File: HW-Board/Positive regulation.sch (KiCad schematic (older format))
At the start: 17 parts, among them Q2 Si4435, U2 MCP4725, U3 AD5245, U4 OP07, U5 INA219POS

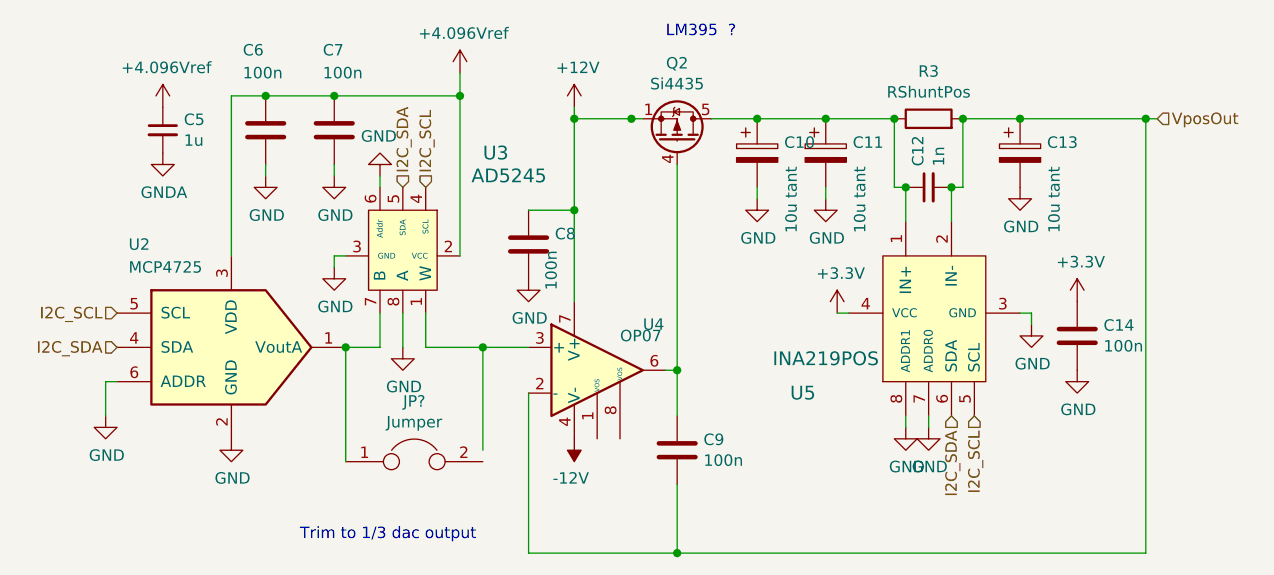
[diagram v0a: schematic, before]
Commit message: sync
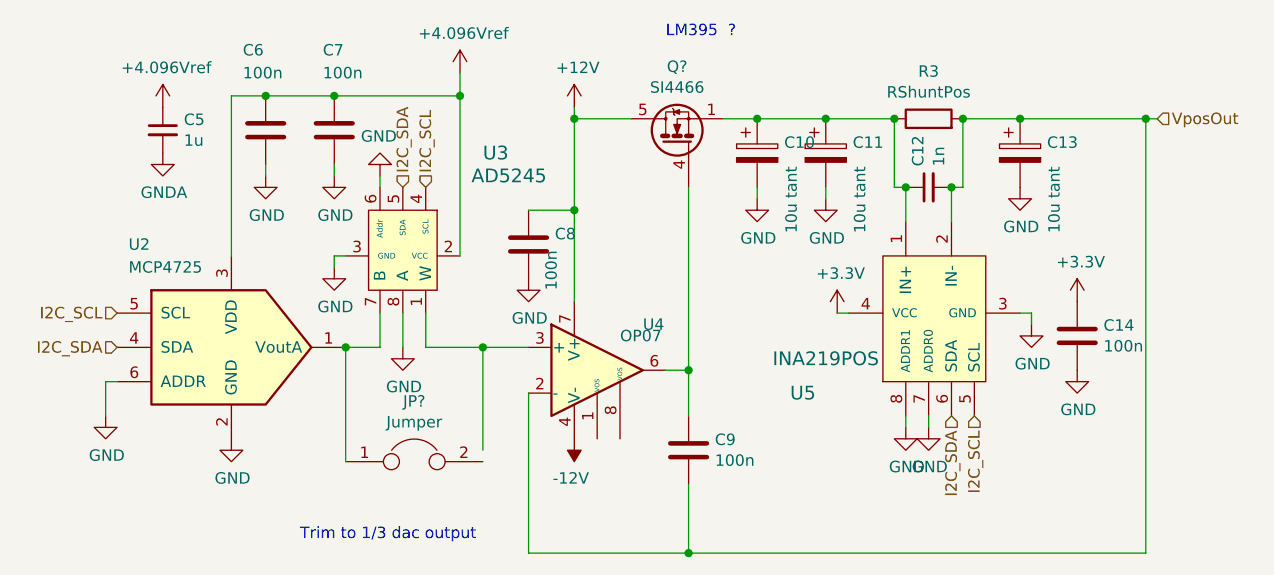
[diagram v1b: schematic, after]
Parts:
- removed Q2: Si4435, Package_SO:SOIC-8_3.9x4.9mm_P1.27mm, symbol BreadbaordPSU-rescue:Si4435-Peters
- added Q?: SI4466, Package_SO:SOIC-8_3.9x4.9mm_P1.27mm, symbol Peters:SI4466
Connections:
- net +12V: now also Q?.5 (D), Q?.6 (D), Q?.7 (D), Q?.8 (D)
- net at C10.1, C11.1, C12.1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: now also Q?.1 (S), Q?.2 (S), Q?.3 (S)
- net at C9.1, U4.6: now also Q?.4 (G)
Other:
- moved on the sheet: C9
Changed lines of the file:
@@
 	5950 2550 5950 2500
 Wire Wire Line
-	6400 3650 6350 3650
+	6450 3650 6350 3650
 Wire Wire Line
 	5750 3750 5750 4450
 Wire Wire Line
-	5750 4450 6400 4450
+	5750 4450 6450 4450
 Wire Wire Line
 	8450 4450 8450 2550
@@
 L Device:C C?
 U 1 1 5CFA023C
-P 6400 4000
+P 6450 4000
 AR Path="/5CFAD453/5CFA023C" Ref="C?"  Part="1"
 AR Path="/5CF8F081/5CFA023C" Ref="C9"  Part="1"
-F 0 "C9" H 6515 4046 50  0000 L CNN
-F 1 "100n" H 6515 3955 50  0000 L CNN
-F 2 "" H 6438 3850 50  0001 C CNN
-F 3 "~" H 6400 4000 50  0001 C CNN
-	1    6400 4000
-	1    0    0    -1
-$EndComp
-Wire Wire Line
-	6400 3850 6400 3650
-Connection ~ 6400 3650
-Wire Wire Line
-	6400 4150 6400 4450
+F 0 "C9" H 6565 4046 50  0000 L CNN
+F 1 "100n" H 6565 3955 50  0000 L CNN
+F 2 "" H 6488 3850 50  0001 C CNN
+F 3 "~" H 6450 4000 50  0001 C CNN
+	1    6450 4000
+	1    0    0    -1
+$EndComp
+Wire Wire Line
+	6450 3850 6450 3650
+Connection ~ 6450 3650
+Wire Wire Line
+	6450 4150 6450 4450
 Wire Wire Line
 	5950 2550 5950 2950
@@
 	3900 3700 3900 3850
 Wire Wire Line
-	6400 4450 8450 4450
-Connection ~ 6400 4450
+	6450 4450 8450 4450
+Connection ~ 6450 4450
 Wire Wire Line
 	7350 2550 7050 2550
@@
 LM395  ?
 Wire Wire Line
-	6400 2750 6400 3650
-Wire Wire Line
-	6550 2550 6750 2550
-Wire Wire Line
-	6200 2550 5950 2550
-Wire Wire Line
-	6250 2550 6200 2550
-Connection ~ 6200 2550
-$Comp
-L BreadbaordPSU-rescue:Si4435-Peters Q?
-U 1 1 5CFA01F0
-P 6400 2650
-AR Path="/5CFAD453/5CFA01F0" Ref="Q?"  Part="1"
-AR Path="/5CF8F081/5CFA01F0" Ref="Q2"  Part="1"
-AR Path="/5CFA01F0" Ref="Q2"  Part="1"
-F 0 "Q2" V 6743 2650 50  0000 C CNN
-F 1 "Si4435" V 6652 2650 50  0000 C CNN
-F 2 "Package_SO:SOIC-8_3.9x4.9mm_P1.27mm" H 6150 2950 50  0001 C CNN
-F 3 "https://www.vishay.com/docs/72123/72123.pdf" H 6250 3050 50  0001 C CNN
-	1    6400 2650
-	0    1    -1   0
-$EndComp
+	6450 2850 6450 3650
 $Comp
 L power:-12V #PWR?
@@
 Wire Wire Line
 	5550 3550 5750 3550
+$Comp
+L Peters:SI4466 Q?
+U 1 1 5D4F6E86
+P 6400 2650
+F 0 "Q?" V 6728 2650 50  0000 C CNN
+F 1 "SI4466" V 6637 2650 50  0000 C CNN
+F 2 "Package_SO:SOIC-8_3.9x4.9mm_P1.27mm" H 6250 2350 50  0001 C CNN
+F 3 "https://www.vishay.com/docs/71820/71820.pdf" H 6150 3000 50  0001 C CNN
+	1    6400 2650
+	0    -1   -1   0
+$EndComp
+Wire Wire Line
+	5950 2550 6200 2550
+Wire Wire Line
+	6600 2550 6750 2550
 $EndSCHEMATC
